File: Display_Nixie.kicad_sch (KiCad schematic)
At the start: 10 parts

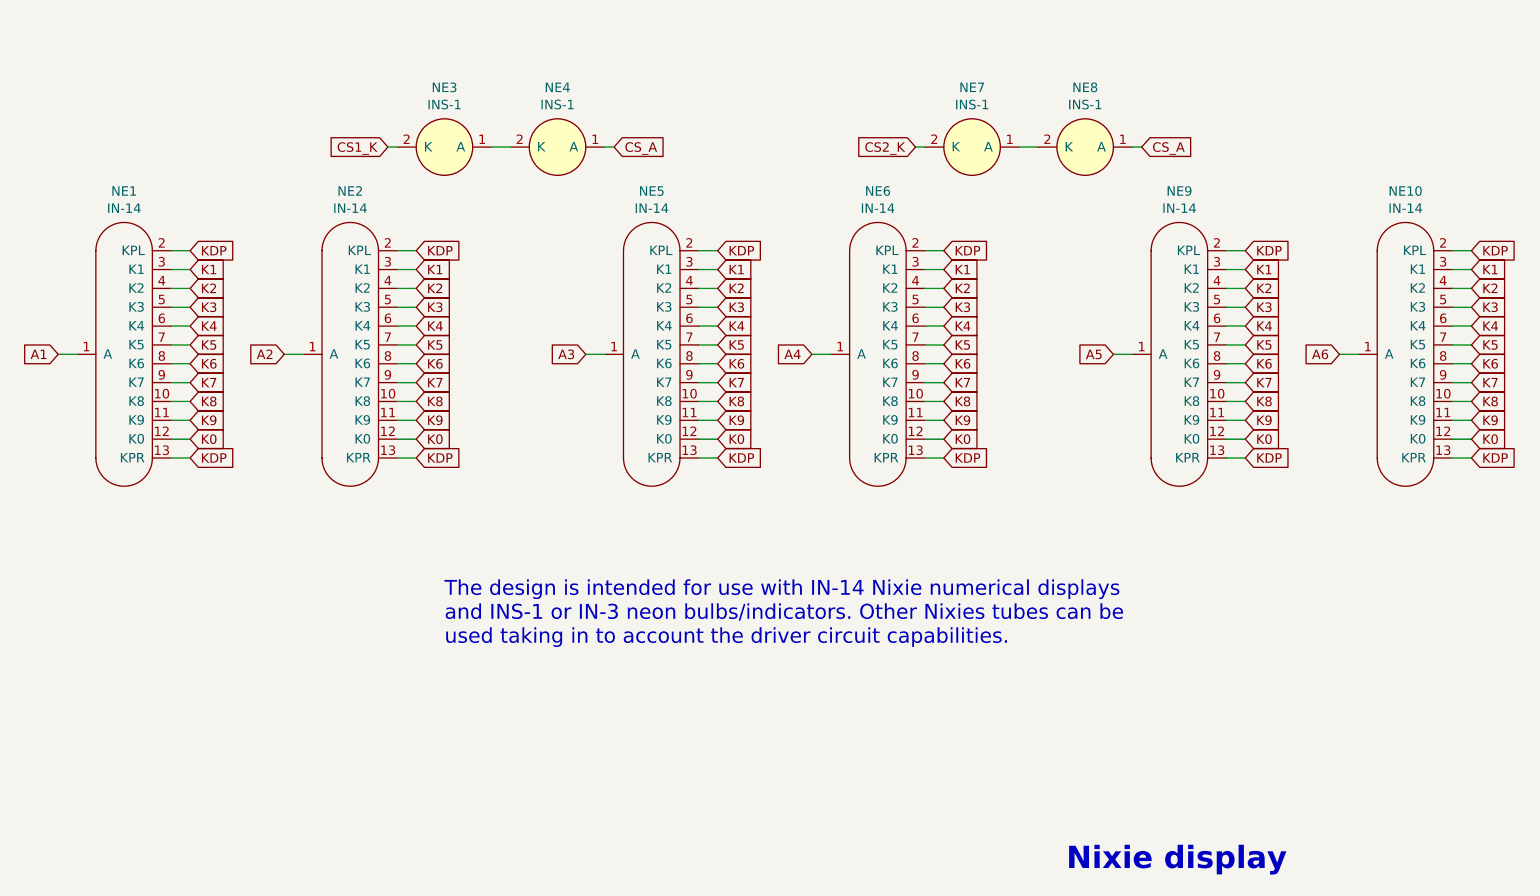
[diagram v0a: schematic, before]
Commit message: WIP
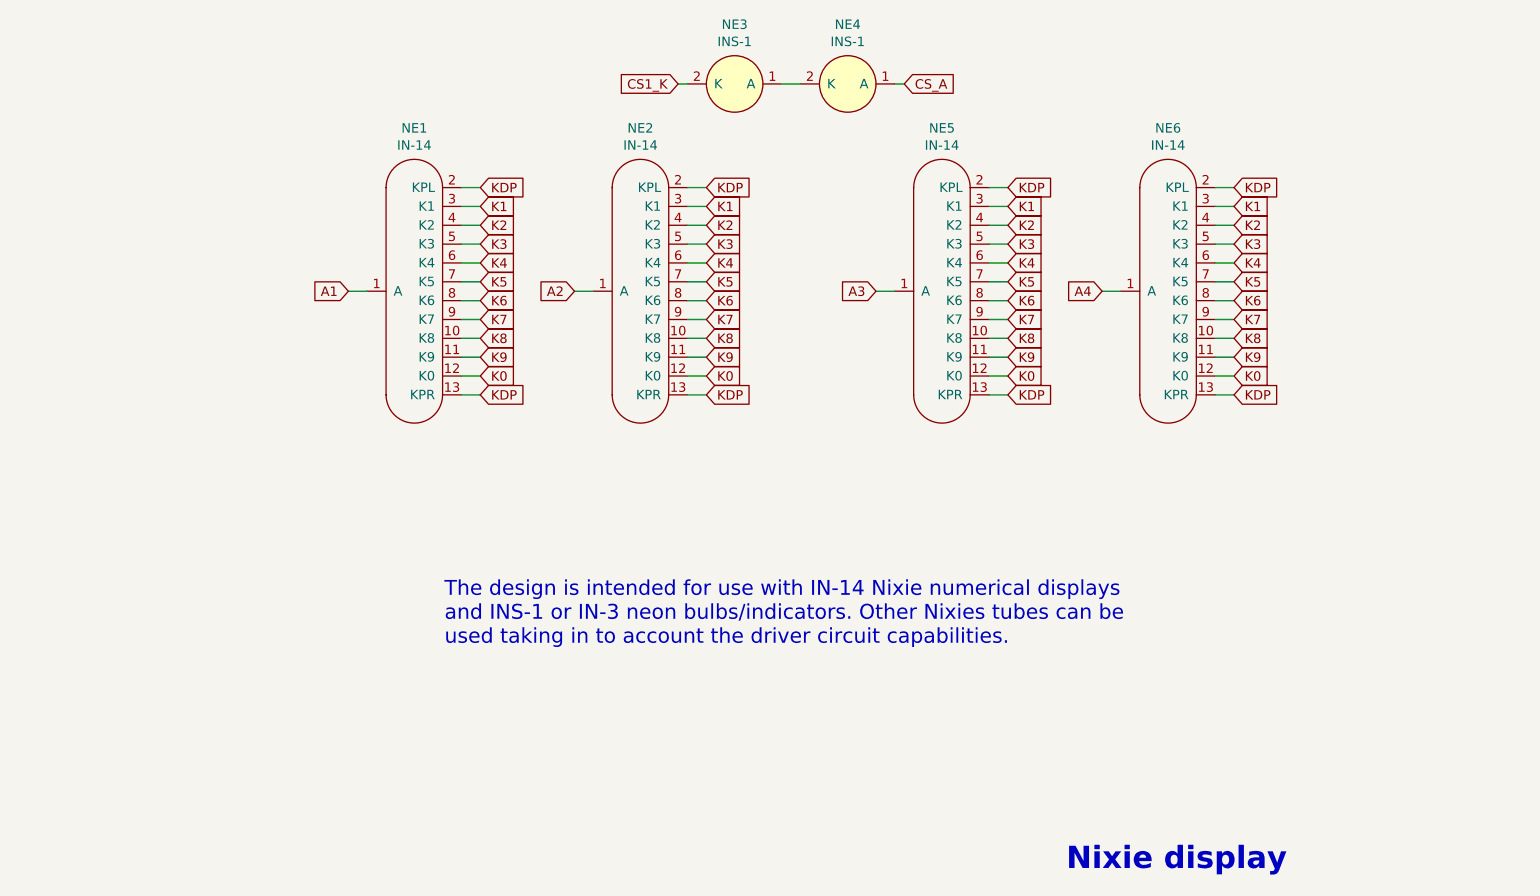
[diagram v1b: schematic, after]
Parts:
- removed NE10, NE9: IN-14, NixieClock:IN-14, symbol NixieClock:IN-14
- removed NE7, NE8: INS-1, Connector_PinSocket_2.54mm:PinSocket_1x02_P2.54mm_Vertical, symbol NixieClock:INS-1
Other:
- moved on the sheet: NE1, NE2, NE3, NE4, NE5, NE6
